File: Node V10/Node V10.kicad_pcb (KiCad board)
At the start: 2 copper layers, 93 x 48 mm, 14 parts, among them J1 Soil Sensor - 1, J2 Soil Sensor - 2, J3 Soil Sensor - 3, J4 Soil Sensor - 4, J5 PiicoDev, J6 Xiao Battery Connectors, U1 MCU, U2 Nano Power Timer

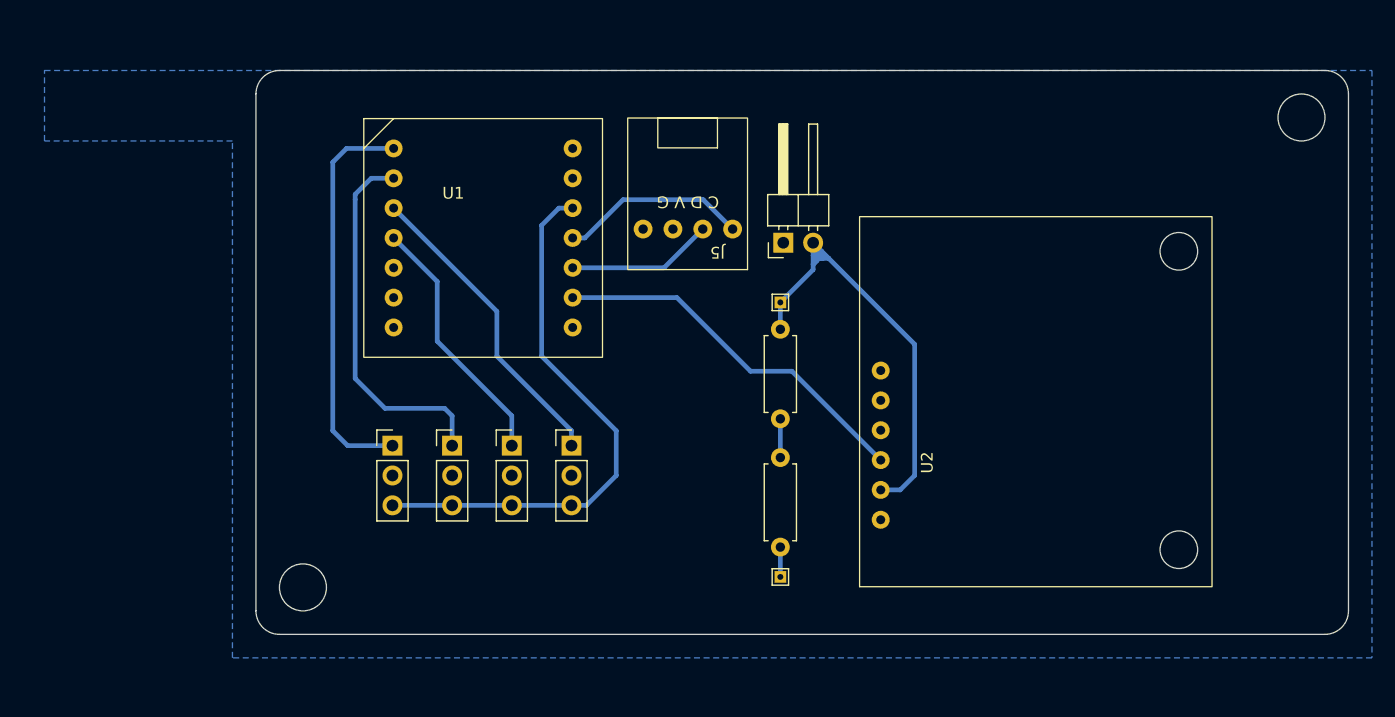
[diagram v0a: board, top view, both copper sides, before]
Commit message: Updates
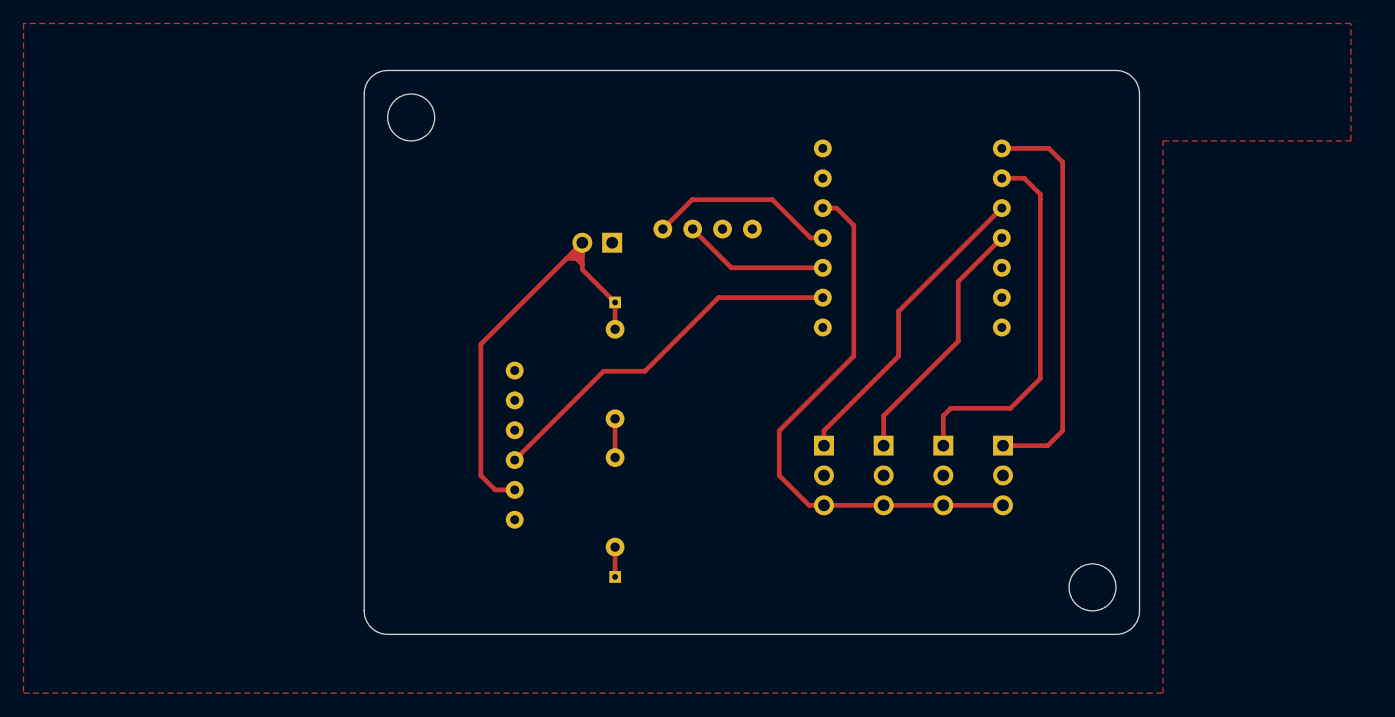
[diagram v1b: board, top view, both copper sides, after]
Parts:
- J1, J2, J3, J4, J5, J6, R1, R2, REF** (x2), TP1, TP2, U1, U2: moved to B.Cu
- moved REF** 75.8 mm to (133.7, 58.4), turned to 180 degrees
- moved REF** 67.2 mm to (191.7, 98.4), turned to 180 degrees
- moved U1 56.9 mm to (186.5, 58.5), turned to 180 degrees
- moved J1 52.0 mm to (184.1, 86.4), turned to 180 degrees
- moved J2 41.8 mm to (179.0, 86.4), turned to 180 degrees
- moved J4 31.7 mm to (173.9, 86.4), turned to 180 degrees
- moved U2 27.6 mm to (144.3, 98.4)
- moved J3 21.5 mm to (168.8, 86.4), turned to 180 degrees
- moved J6 14.6 mm to (150.8, 69.1)
- moved R1 14.1 mm to (151.0, 76.5)
- moved R2 14.1 mm to (151.0, 87.4)
- moved TP1 14.1 mm to (151.0, 97.5)
- moved TP2 14.1 mm to (151.0, 74.2)
- moved J5 8.48 mm to (153.8, 71.4), turned to 0 degrees
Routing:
- added copper zone on F.Cu, net GND
- removed copper zone on B.Cu, net GND
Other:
- board size 93 x 48 mm -> 66 x 48 mm
